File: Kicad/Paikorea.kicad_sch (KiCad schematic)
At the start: 54 parts, among them J1 AudioJack3, J2 TPS43-201A-S, J3 TPS43-201A-S, J4 AudioJack3, K10 PG1316S, K11 PG1316S, K12 PG1316S, K13 PG1316S, K14 PG1316S, K15 PG1316S, K16 PG1316S, K17 PG1316S, K18 PG1316S, K19 PG1316S, K20 PG1316S, K21 PG1316S, K22 PG1316S, K4 PG1316S, K5 PG1316S, K6 PG1316S, K7 PG1316S, K8 PG1316S, K9 PG1316S, U1 RP2040-Zero, U2 RP2040-Zero

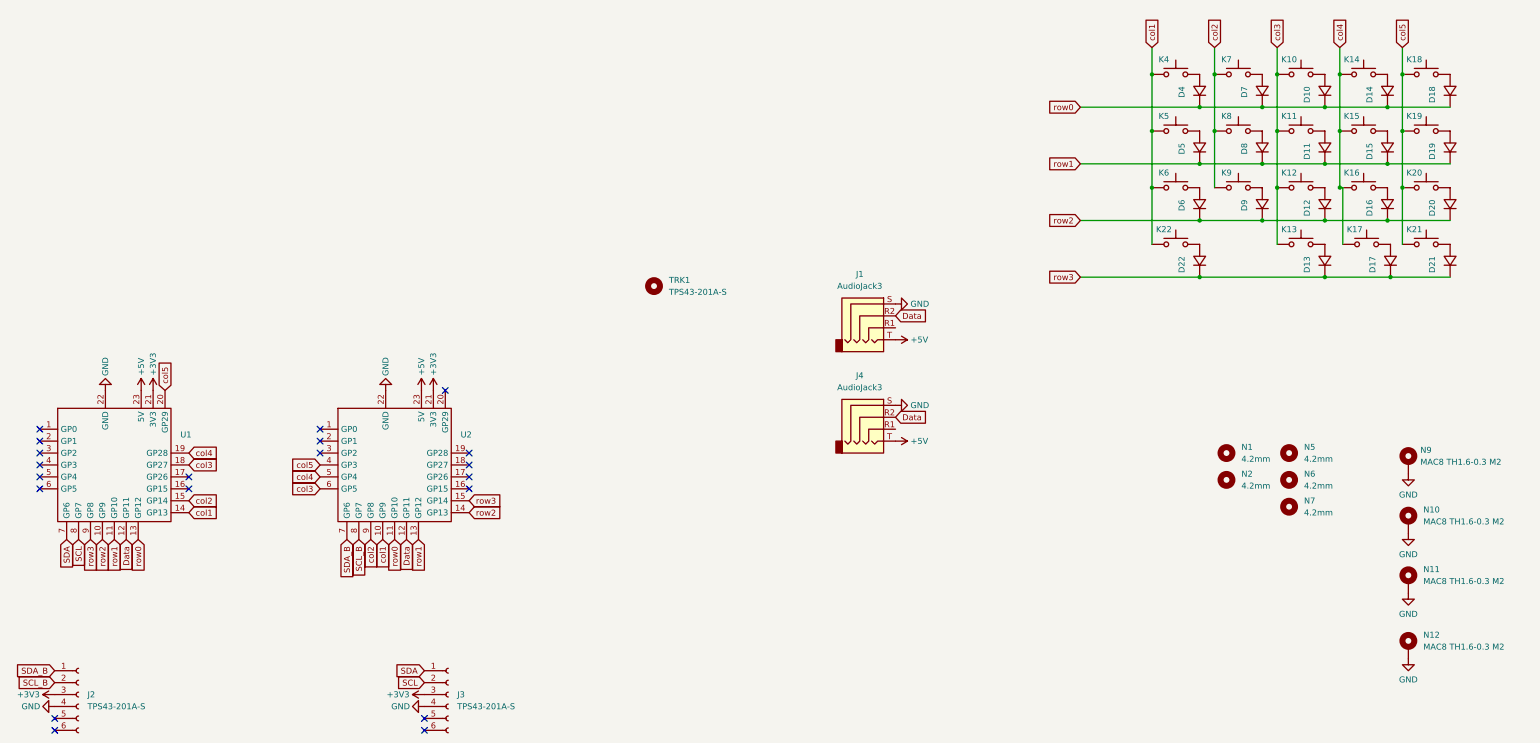
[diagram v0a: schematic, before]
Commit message: .
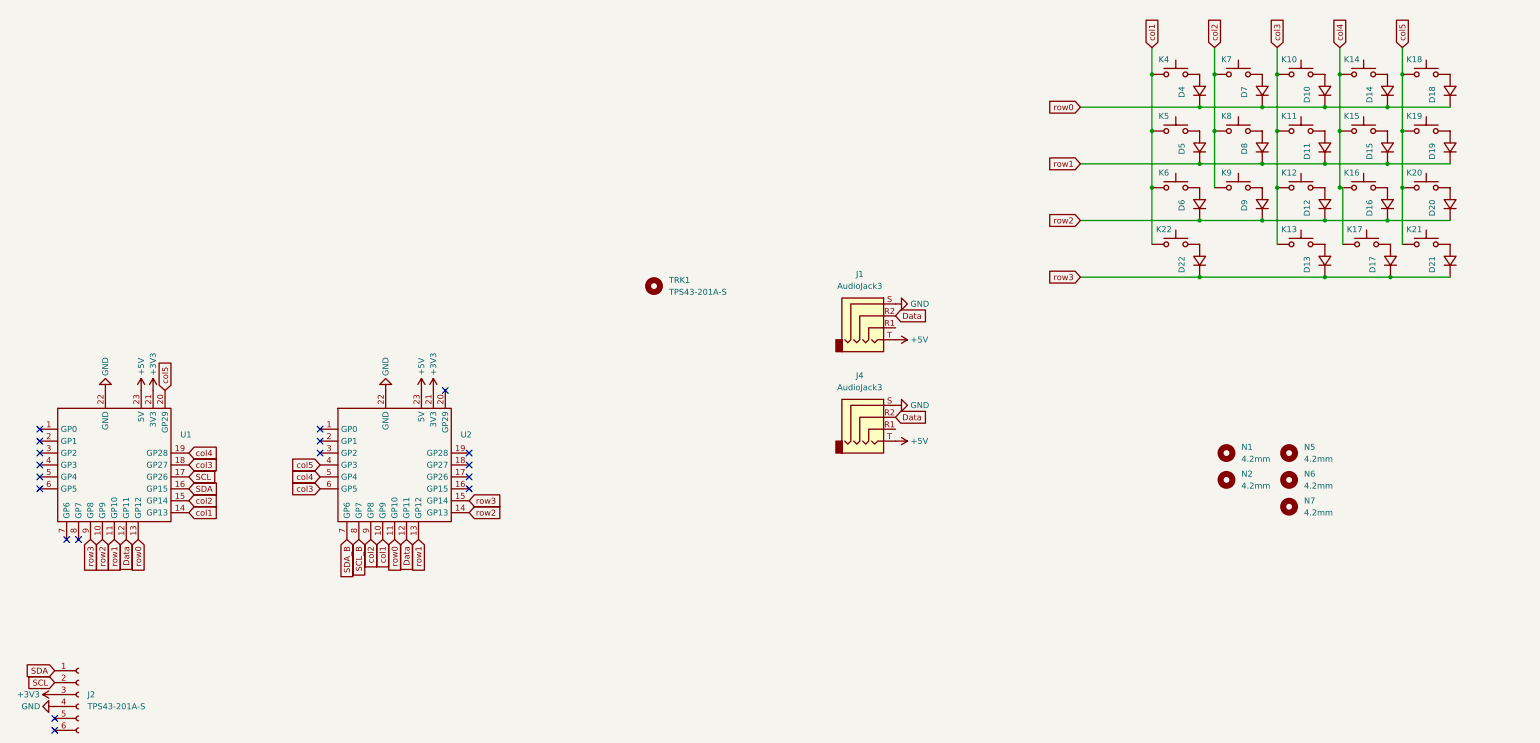
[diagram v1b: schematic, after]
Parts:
- removed J3: TPS43-201A-S, DreaM117er-keebLibrary:Hirose_FH12-6S-0.5SH_1x06-1MP_P0.50mm_Horizontal, symbol Connector:Conn_01x06_Socket
- removed N10, N11, N12, N9: MAC8 TH1.6-0.3 M2, DreaM117er-keebLibrary:MAC8_TH0816-XX-M2-Dual_Pad, symbol Mechanical:MountingHole_Pad
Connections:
- net SCL: now also J2.2 (Pin_2), U1.17 (GP26); no longer U1.8 (GP7)
- net SCL_B: no longer J2.2 (Pin_2)
- net SDA: now also J2.1 (Pin_1), U1.16 (GP15); no longer U1.7 (GP6)
- net SDA_B: no longer J2.1 (Pin_1)
- no-connect marks 20 -> 18
